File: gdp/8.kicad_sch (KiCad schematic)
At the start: 12 parts, among them IC13 74LS244, IC16 74LS245, IC4 74LS367, IC5 SCN2674

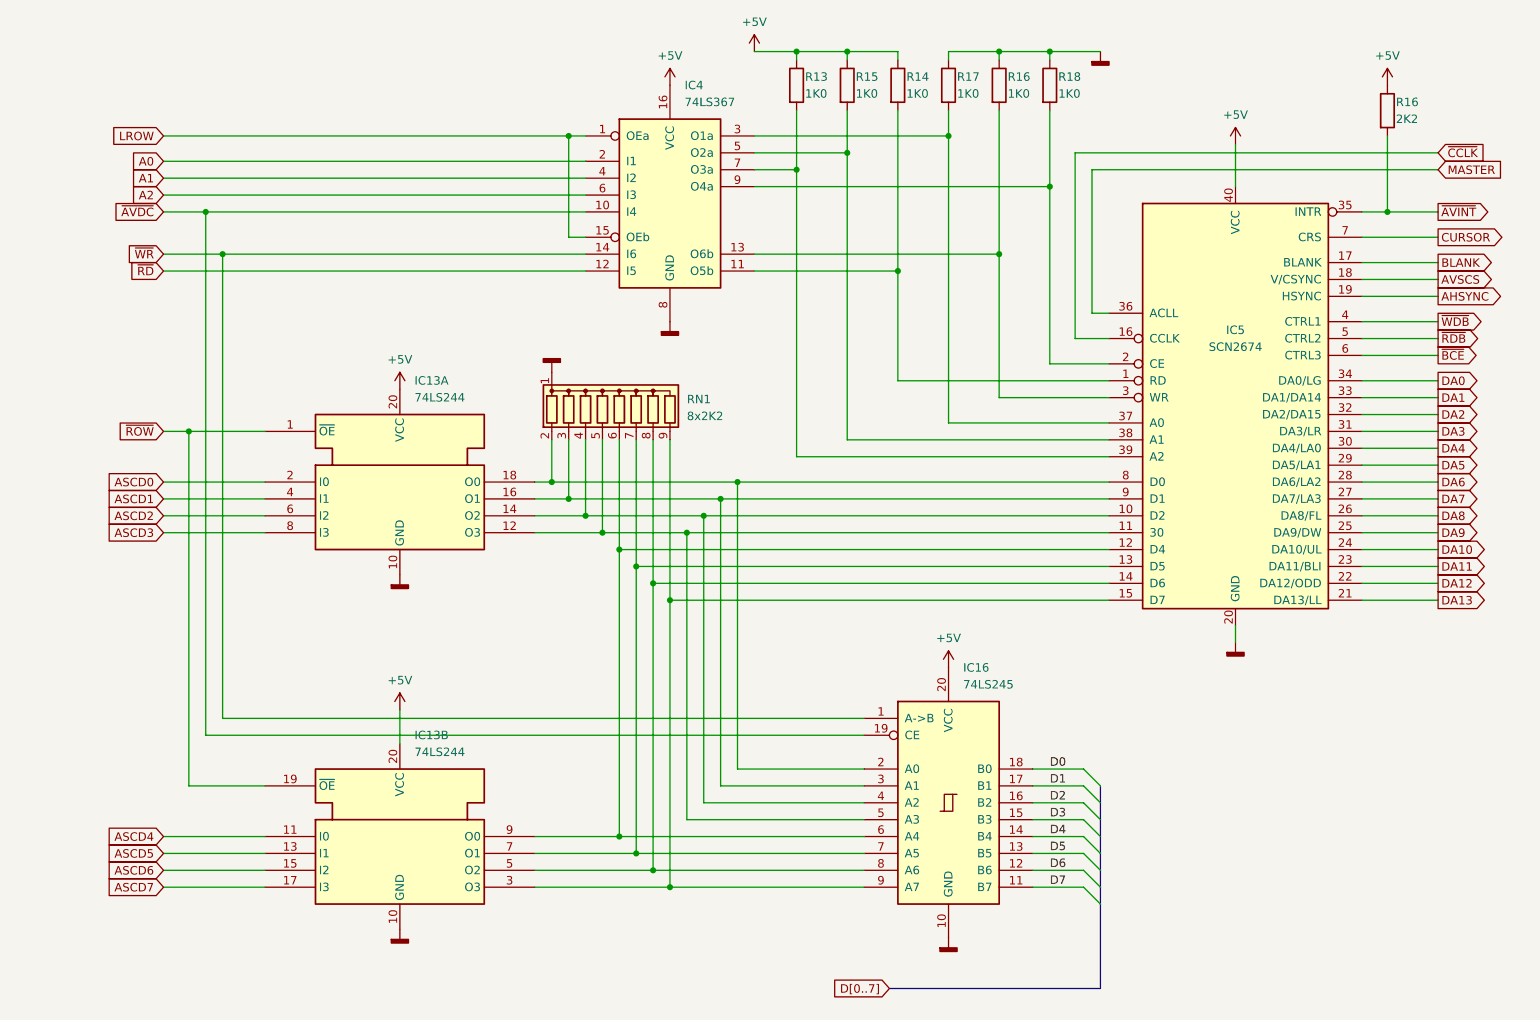
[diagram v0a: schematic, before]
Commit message: Adds Sheet 12
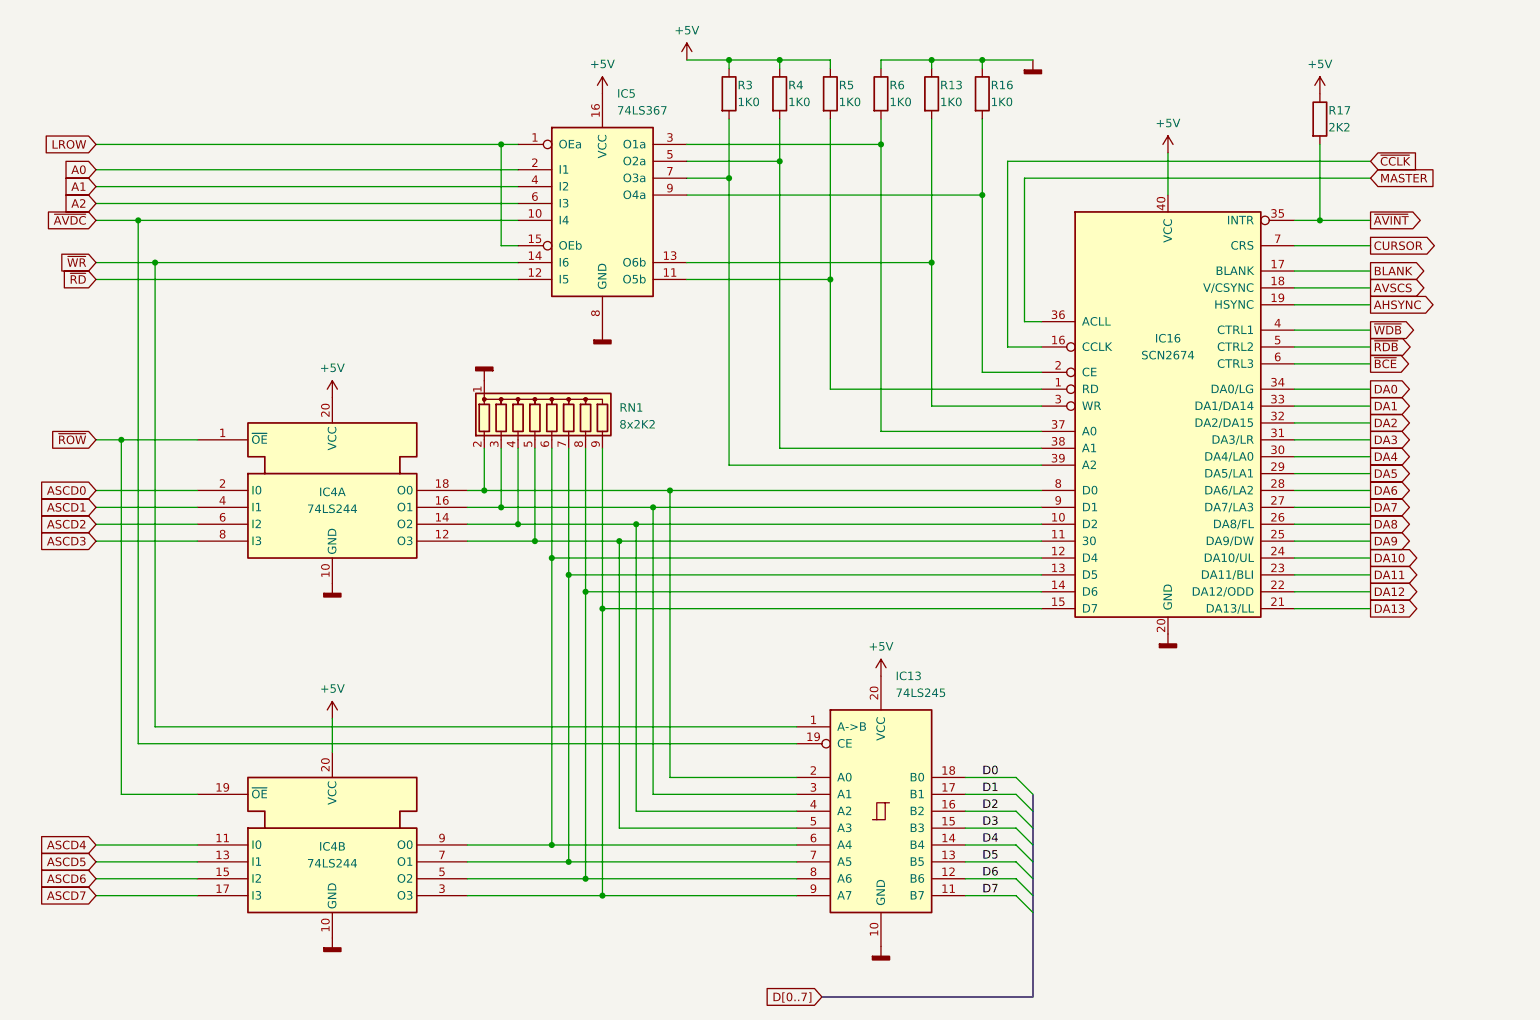
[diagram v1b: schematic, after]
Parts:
- removed IC13: 74LS244, symbol 74xx_IEEE:74LS244
- removed IC16: 74LS245, symbol 74xx:74LS245
- removed IC4: 74LS367, symbol 74xx:74LS367
- removed IC5: SCN2674, Package_DIP:DIP-40_W15.24mm, symbol MCU_Parallax:P8X32A-D40
- removed R14, R15, R16, R18: 1K0, symbol Device:R
- removed R16: 2K2, symbol Device:R
- added IC13: 74LS245, symbol 74xx:74LS245
- added IC16: SCN2674, Package_DIP:DIP-40_W15.24mm, symbol MCU_Parallax:P8X32A-D40
- added IC4: 74LS244, symbol 74xx_IEEE:74LS244
- added IC5: 74LS367, symbol 74xx:74LS367
- added R16, R3, R4, R5, R6: 1K0, symbol Device:R
- R17: value 1K0 -> 2K2
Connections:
- net +5V: now also R17.1, IC13.20 (VCC), IC16.40 (VCC), IC4.20 (VCC), IC4.20 (VCC), IC5.16 (VCC), R3.1, R4.1, R5.1; no longer R13.1
- net A0: now also IC5.2 (I1)
- net A1: now also IC5.4 (I2)
- net A2: now also IC5.6 (I3)
- net AHSYNC: now also IC16.19 (HSYNC)
- net ASCD0: now also IC4.2 (I0)
- net ASCD1: now also IC4.4 (I1)
- net ASCD2: now also IC4.6 (I2)
- net ASCD3: now also IC4.8 (I3)
- net ASCD4: now also IC4.11 (I0)
- net ASCD5: now also IC4.13 (I1)
- net ASCD6: now also IC4.15 (I2)
- net ASCD7: now also IC4.17 (I3)
- net AVSCS: now also IC16.18 (V/CSYNC)
- net BLANK: now also IC16.17 (BLANK)
- net CURSOR: now also IC16.7 (CRS)
- net D0: now also IC13.18 (B0)
- net D1: now also IC13.17 (B1)
- net D2: now also IC13.16 (B2)
- net D3: now also IC13.15 (B3)
- net D4: now also IC13.14 (B4)
- net D5: now also IC13.13 (B5)
- net D6: now also IC13.12 (B6)
- net D7: now also IC13.11 (B7)
- net DA0: now also IC16.34 (DA0/LG)
- net DA1: now also IC16.33 (DA1/DA14)
- net DA10: now also IC16.24 (DA10/UL)
- net DA11: now also IC16.23 (DA11/BLI)
- net DA12: now also IC16.22 (DA12/ODD)
- net DA13: now also IC16.21 (DA13/LL)
- net DA2: now also IC16.32 (DA2/DA15)
- net DA3: now also IC16.31 (DA3/LR)
- net DA4: now also IC16.30 (DA4/LA0)
- net DA5: now also IC16.29 (DA5/LA1)
- net DA6: now also IC16.28 (DA6/LA2)
- net DA7: now also IC16.27 (DA7/LA3)
- net DA8: now also IC16.26 (DA8/FL)
- net DA9: now also IC16.25 (DA9/DW)
- net GNDD: now also R13.1, IC13.10 (GND), IC16.20 (GND), IC4.10 (GND), IC4.10 (GND), IC5.8 (GND), R16.1, R6.1; no longer R17.1
- net LROW: now also IC5.1 (OEa), IC5.15 (OEb)
- net MASTER: now also IC16.36 (ACLL)
- net ~{AVDC}: now also IC13.19 (CE), IC5.10 (I4)
- net ~{AVINT}: now also R17.2, IC16.35 (INTR)
- net ~{BCE}: now also IC16.6 (CTRL3)
- net ~{CCLK}: now also IC16.16 (CCLK)
- net ~{RDB}: now also IC16.5 (CTRL2)
- net ~{RD}: now also IC5.12 (I5)
- net ~{ROW}: now also IC4.1 (~{OE}), IC4.19 (~{OE})
- net ~{WDB}: now also IC16.4 (CTRL1)
- net ~{WR}: now also IC13.1 (A->B), IC5.14 (I6)
- net at R13.2: now also IC16.3 (WR), IC5.13 (O6b)
- net at RN1.9 (R8): now also IC13.9 (A7), IC16.15 (D7), IC4.3 (O3)
- net at RN1.8 (R7): now also IC13.8 (A6), IC16.14 (D6), IC4.5 (O2)
- net at RN1.7 (R6): now also IC13.7 (A5), IC16.13 (D5), IC4.7 (O1)
- net at RN1.6 (R5): now also IC13.6 (A4), IC16.12 (D4), IC4.9 (O0)
- net at RN1.2 (R1): now also IC13.2 (A0), IC16.8 (D0), IC4.18 (O0)
- net at RN1.3 (R2): now also IC13.3 (A1), IC16.9 (D1), IC4.16 (O1)
- net at RN1.4 (R3): now also IC13.4 (A2), IC16.10 (D2), IC4.14 (O2)
- net at RN1.5 (R4): now also IC13.5 (A3), IC16.11 (30), IC4.12 (O3)
- new net: IC16.2 (CE), IC5.9 (O4a), R16.2
- new net: IC16.39 (A2), IC5.7 (O3a), R3.2
- new net: IC16.1 (RD), IC5.11 (O5b), R5.2
- new net: IC16.37 (A0), IC5.3 (O1a), R6.2
- new net: IC16.38 (A1), IC5.5 (O2a), R4.2
